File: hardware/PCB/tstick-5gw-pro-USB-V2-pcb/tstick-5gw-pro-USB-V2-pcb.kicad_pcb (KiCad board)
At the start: 4 copper layers, 57.2 x 25.4 mm, 63 parts, among them J1 USB_C_Receptacle_USB2.0, Q1 BSS138, Q2 BSS138, Q3 BSS138, SW1 JST-SH-1.00mm 1x2, SW2 PTS810 SJM Switch, SW3 PTS810 SJM Switch, U1 USBLC6-2P6, U2 MCP73871, U3 NCP167AMX330TBG, U4 NCP167AMX180TBG

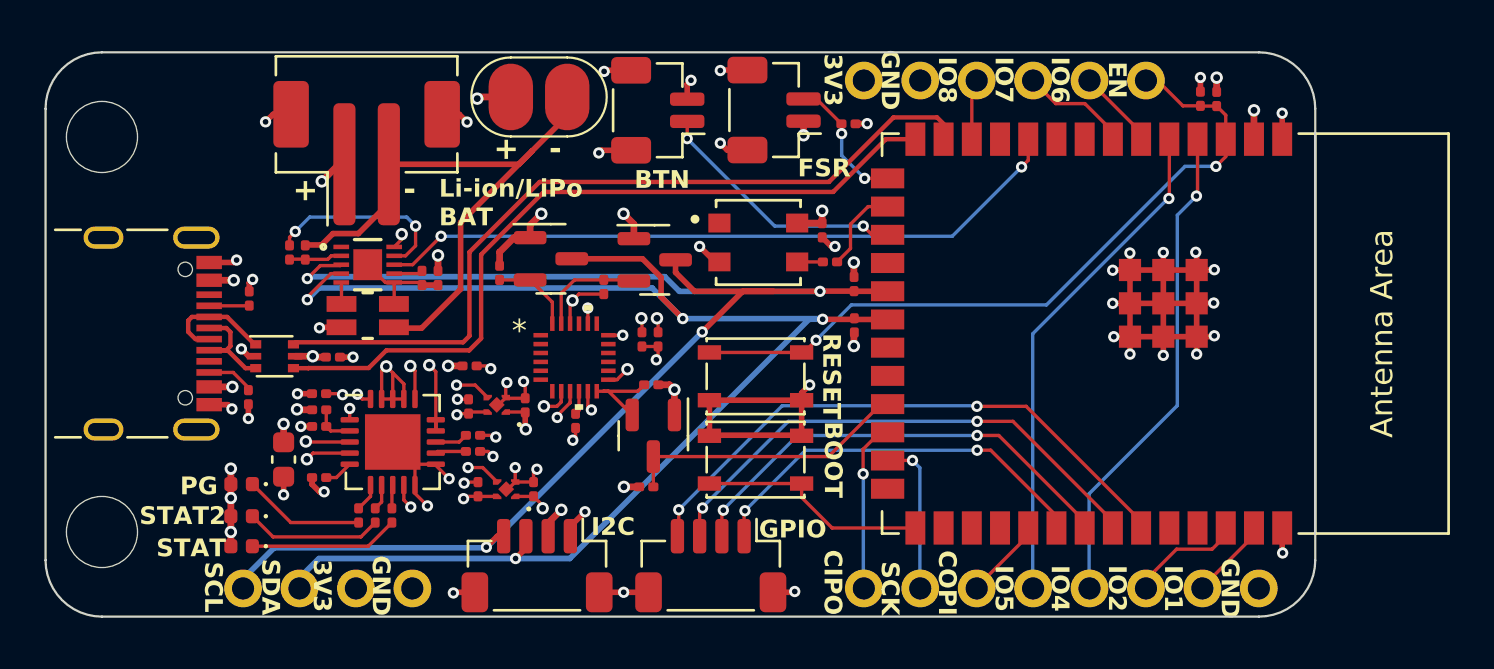
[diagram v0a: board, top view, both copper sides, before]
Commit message: added up to date manufacturing files
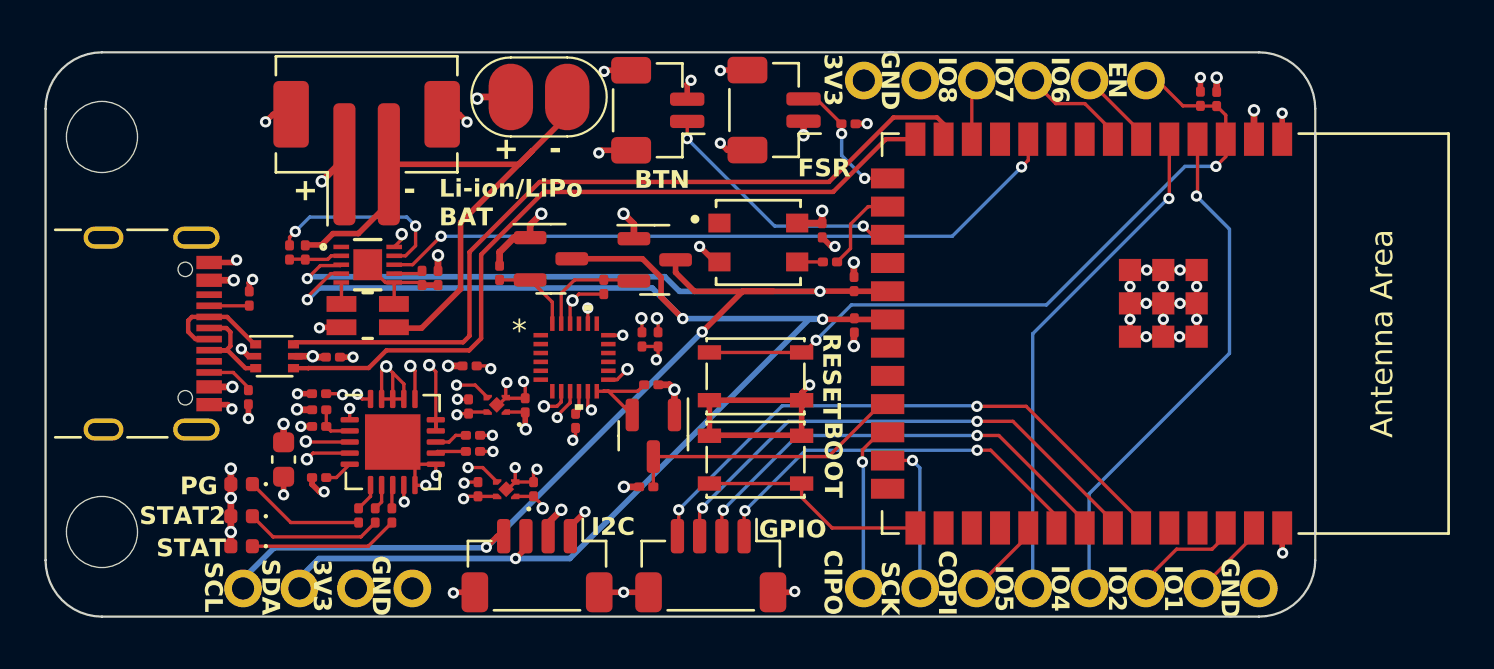
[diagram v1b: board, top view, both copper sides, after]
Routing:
- net GND: track 89.1 -> 87.0 mm
- net /IO4: track 21.9 -> 23.1 mm
